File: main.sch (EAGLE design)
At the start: 32 parts, among them IC1 4050D, U1 MCP2551, U2 STN1110

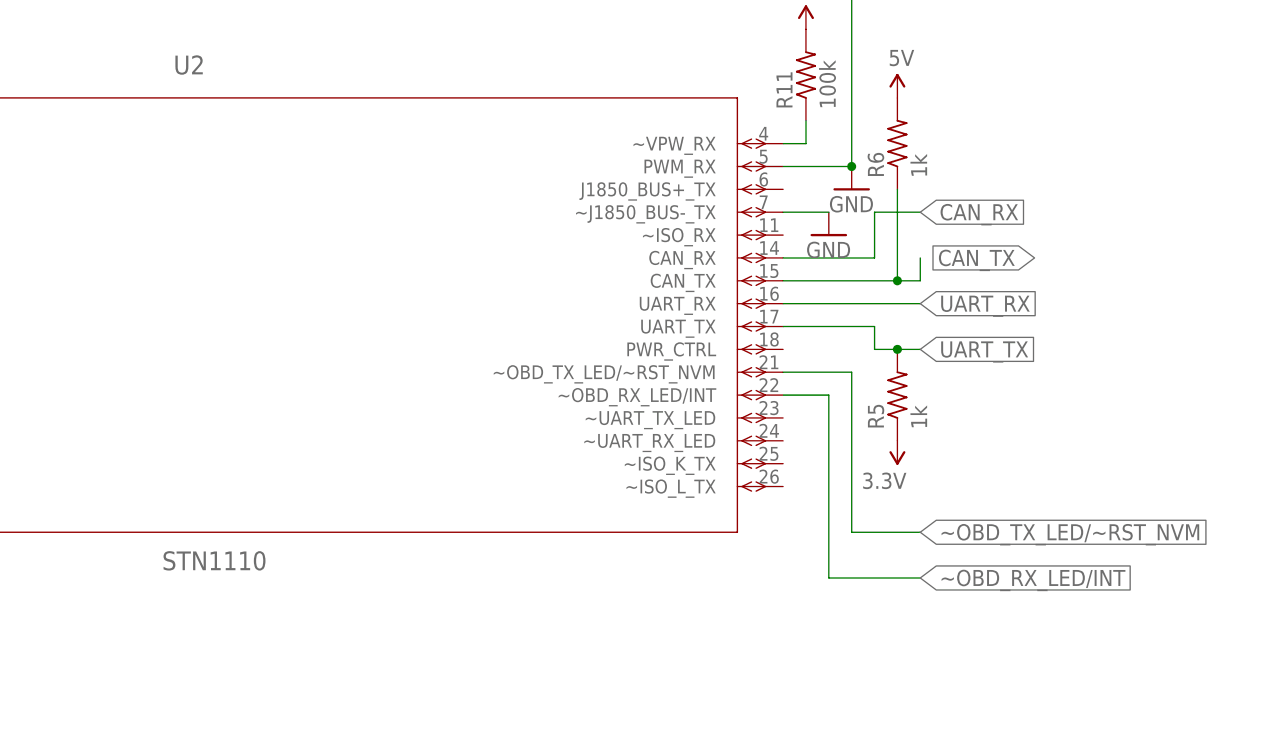
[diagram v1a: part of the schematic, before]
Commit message: Review phase 1
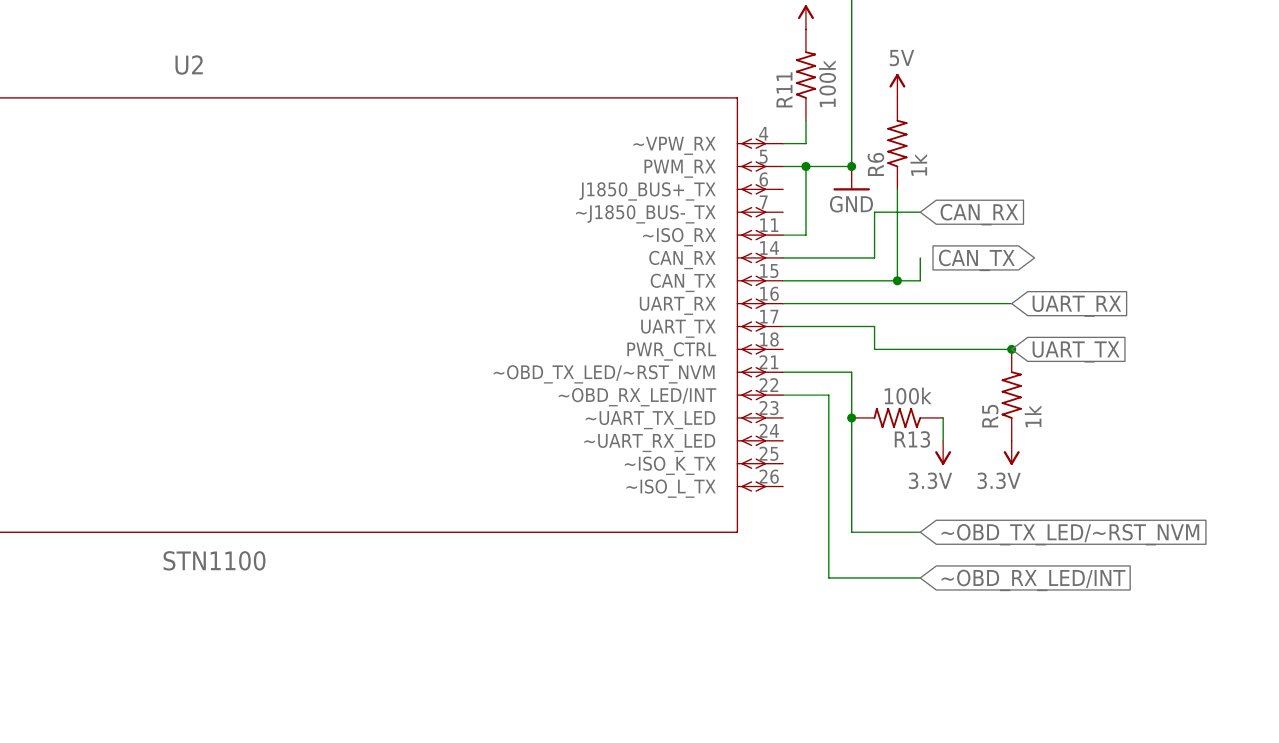
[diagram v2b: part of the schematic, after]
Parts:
- added R13: 100k, resistor:R-US_0204/7
- U2: value STN1110 -> STN1100
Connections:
- net 3.3V: now also R13.1
- net GND: now also U2.~ISO_RX; no longer U2.~J1850_BUS-_TX
- net ~OBD_TX_LED/~RST_NVM: now also R13.2
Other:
- moved on the sheet: R5
